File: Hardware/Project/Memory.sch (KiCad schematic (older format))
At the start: 3 parts, among them U10 28C256, U12 28C256, U18 74LS138

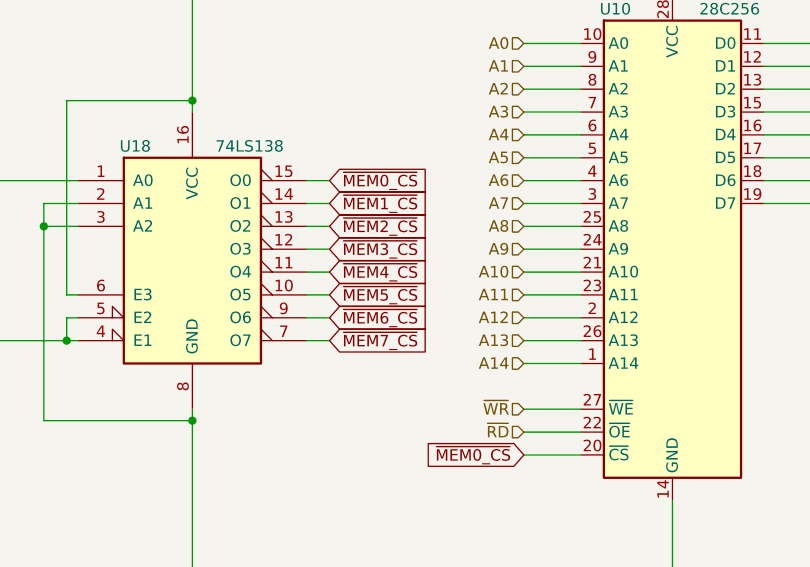
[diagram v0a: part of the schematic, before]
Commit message: 1
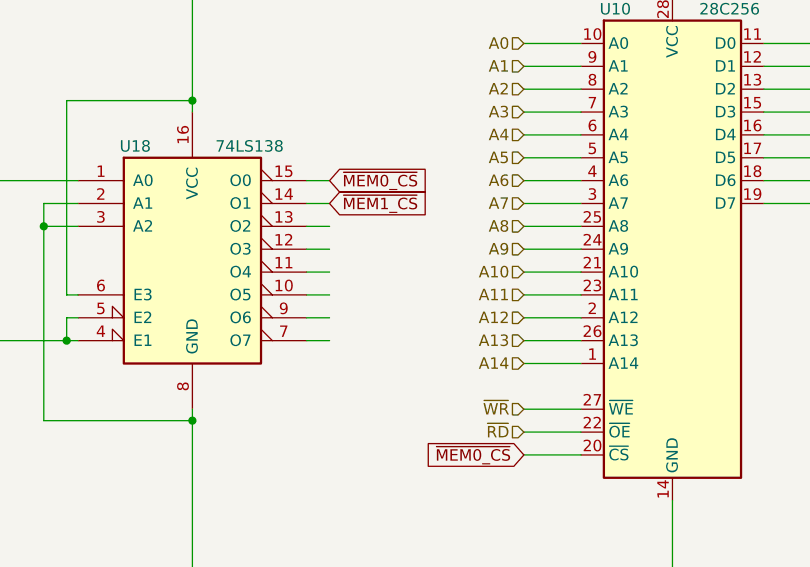
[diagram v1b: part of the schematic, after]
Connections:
- net labels removed: ~MEM2_CS, ~MEM3_CS, ~MEM4_CS, ~MEM5_CS, ~MEM6_CS, ~MEM7_CS
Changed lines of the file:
@@
 $Descr A4 11693 8268
 encoding utf-8
-Sheet 5 6
+Sheet 4 6
 Title ""
 Date ""
@@
 Wire Wire Line
 	3350 2650 3250 2650
-Text GLabel 3350 2750 2    50   Input ~ 0
-~MEM2_CS
 Wire Wire Line
 	3350 2750 3250 2750
-Text GLabel 3350 2850 2    50   Input ~ 0
-~MEM3_CS
 Wire Wire Line
 	3350 2850 3250 2850
-Text GLabel 3350 2950 2    50   Input ~ 0
-~MEM4_CS
 Wire Wire Line
 	3350 2950 3250 2950
-Text GLabel 3350 3050 2    50   Input ~ 0
-~MEM5_CS
 Wire Wire Line
 	3350 3050 3250 3050
-Text GLabel 3350 3150 2    50   Input ~ 0
-~MEM6_CS
 Wire Wire Line
 	3350 3150 3250 3150
-Text GLabel 3350 3250 2    50   Input ~ 0
-~MEM7_CS
 Wire Wire Line
 	3350 3250 3250 3250
